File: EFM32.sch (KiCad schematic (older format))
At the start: 9 parts, among them J5 MCU_debug, J6 67997-410HLF, U7 EFM32GG11B4xx, Y1 48Mhz

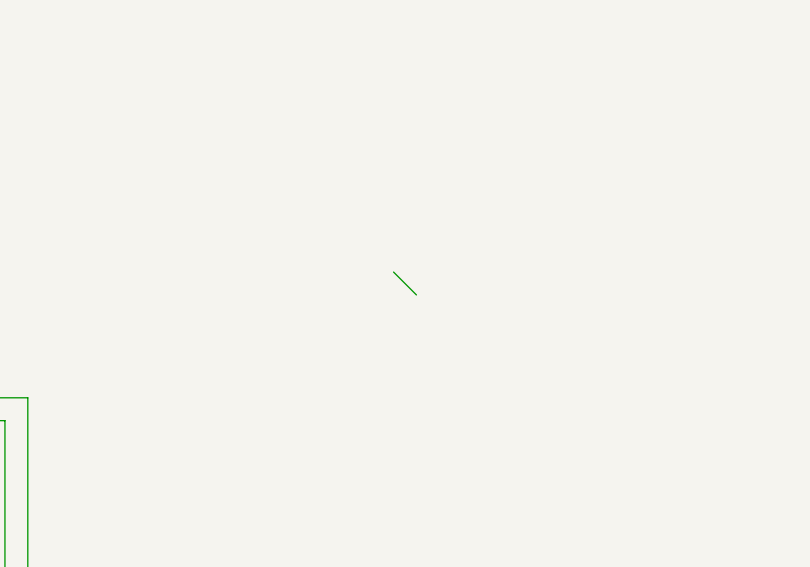
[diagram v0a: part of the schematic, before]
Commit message: Rearrange and wire most of PCB FOR REAL THIS TIME
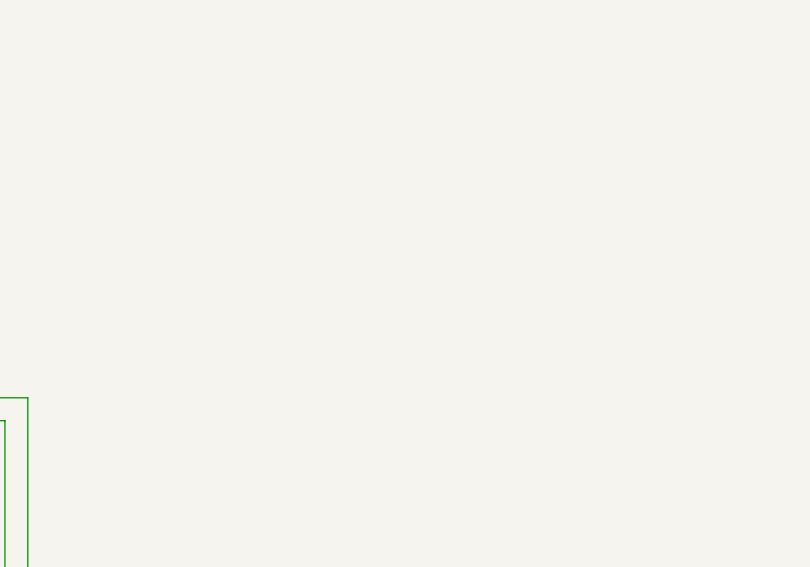
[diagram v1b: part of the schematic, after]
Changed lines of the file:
@@
 Wire Wire Line
 	2300 3900 4100 3900
-Entry Wire Line
-	10100 6050 10200 6150
 Text HLabel 4300 6700 0    50   UnSpc ~ 0
 USB_D+

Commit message: Fix a few more noclipping objects and labels
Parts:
- J6: value 67997-410HLF -> MCU_GPIO
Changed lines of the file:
@@
 P 6750 6750
 F 0 "J6" H 7400 7237 60  0000 C CNN
-F 1 "67997-410HLF" H 7400 7131 60  0000 C CNN
+F 1 "MCU_GPIO" H 7400 7131 60  0000 C CNN
 F 2 "footprints:67997-410HLF" H 7400 7090 60  0001 C CNN
 F 3 "" H 6750 6900 60  0000 C CNN
